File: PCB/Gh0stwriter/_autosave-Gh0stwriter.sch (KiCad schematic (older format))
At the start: 20 parts, among them J1 Conn_01x06, J2 Conn_01x02, J3 Conn_01x06, J4 Conn_01x02, J5 Conn_01x06, J6 Conn_01x06, J7 Conn_01x02, Q1 Q_NPN_Darlington_ECB

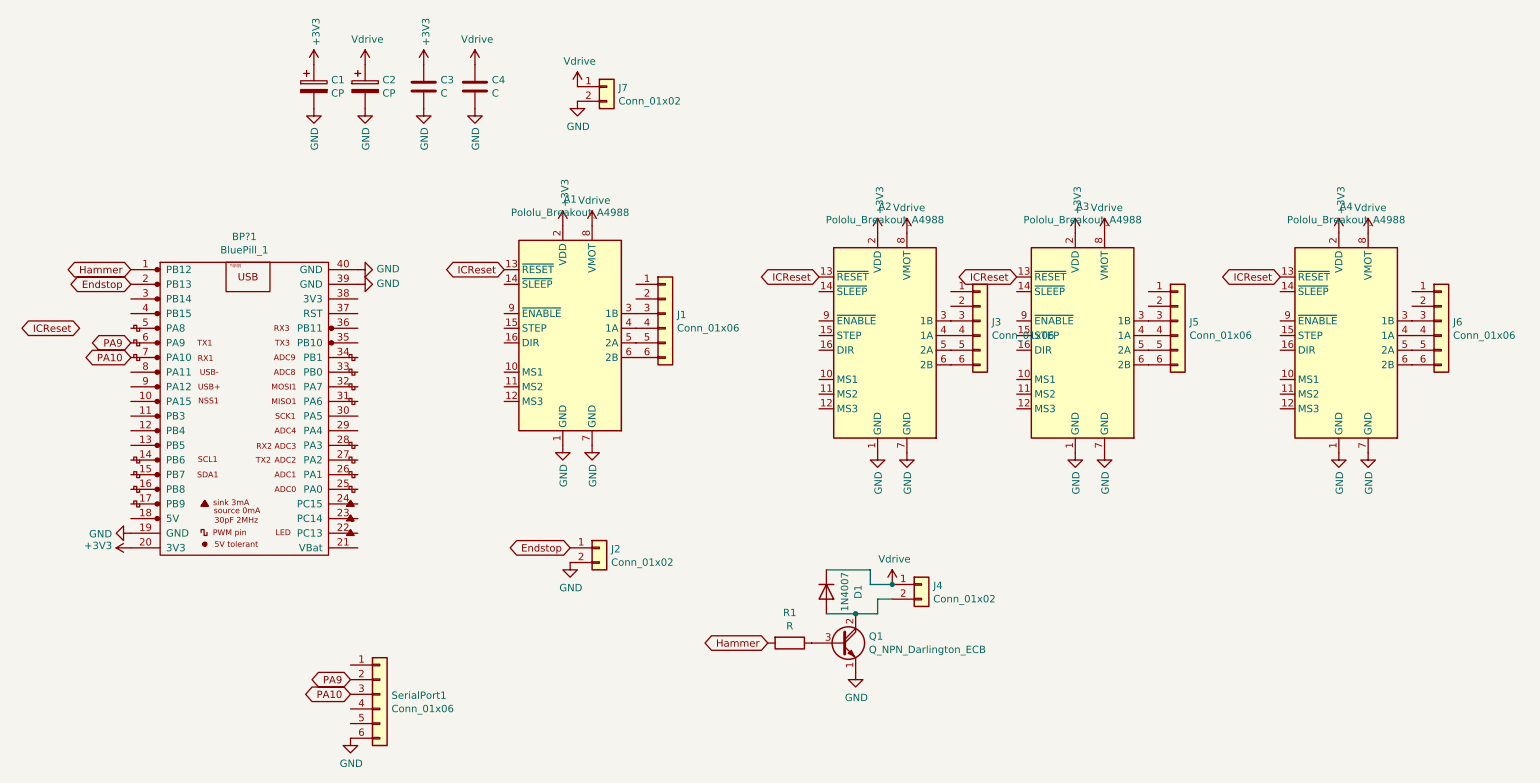
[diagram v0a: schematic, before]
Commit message: Finished first Version of the pcb
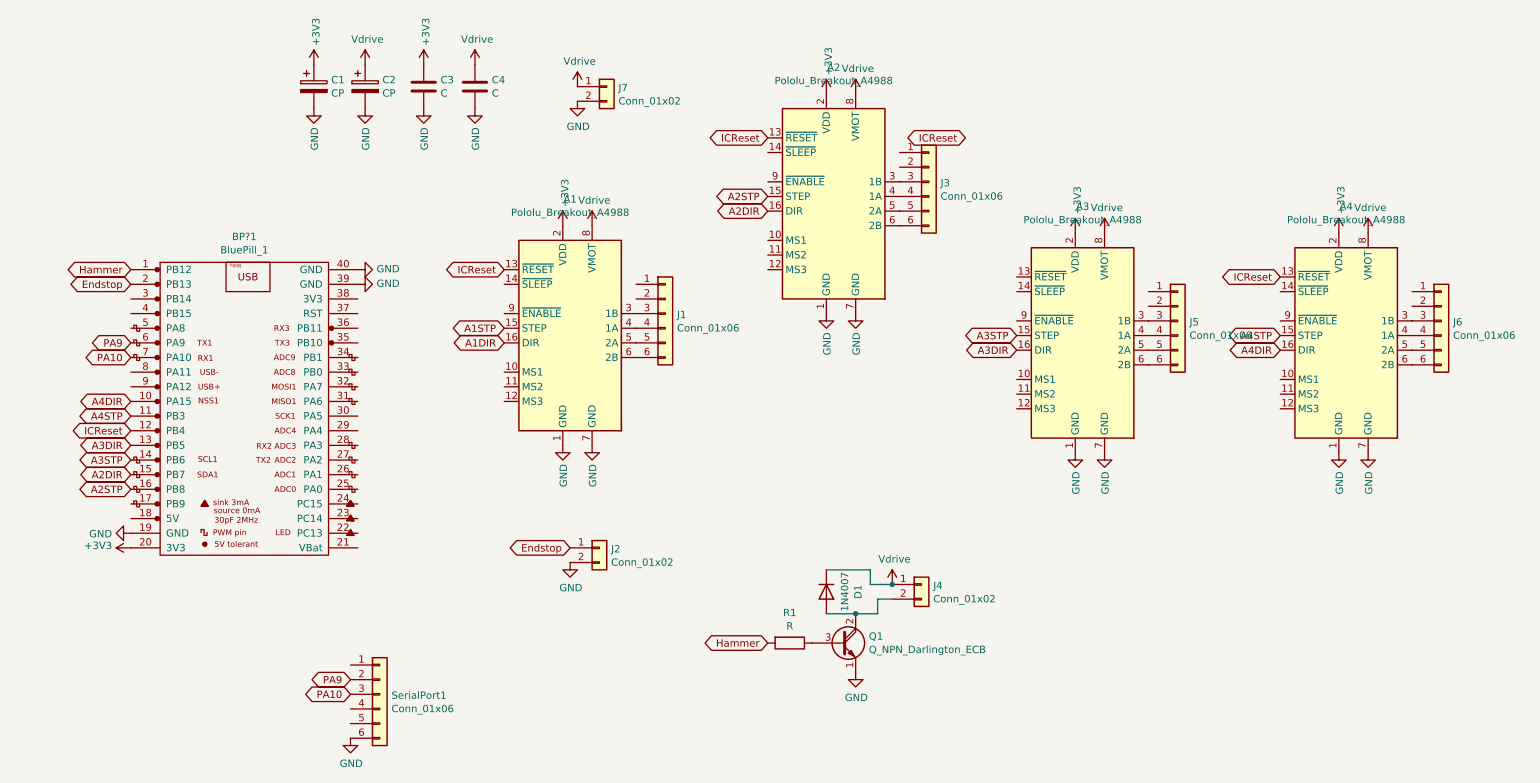
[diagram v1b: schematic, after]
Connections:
- net ICReset: now also BP?1.12 (PB4); no longer A3.13 (~RESET)
- net A3STP: now reaches A3.15 (STEP)
- net A3STP: now also BP?1.14 (PB6)
- net A3DIR: now reaches A3.16 (DIR)
- net A3DIR: now also BP?1.13 (PB5)
- net A4DIR: now reaches BP?1.10 (PA15)
- net A4DIR: now also A4.16 (DIR)
- net A4STP: now reaches BP?1.11 (PB3)
- net A4STP: now also A4.15 (STEP)
- net A2DIR: now reaches BP?1.15 (PB7)
- net A2DIR: now also A2.16 (DIR)
- net A2STP: now reaches BP?1.16 (PB8)
- net A2STP: now also A2.15 (STEP)
- net A1STP: now reaches A1.15 (STEP)
- net A1DIR: now reaches A1.16 (DIR)
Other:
- moved on the sheet: A2, J3
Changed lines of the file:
@@
 L Driver_Motor:Pololu_Breakout_A4988 A2
 U 1 1 5ECFA6AE
-P 6250 4250
-F 0 "A2" H 6300 5131 50  0000 C CNN
-F 1 "Pololu_Breakout_A4988" H 6300 5040 50  0000 C CNN
-F 2 "Module:Pololu_Breakout-16_15.2x20.3mm" H 6525 3500 50  0001 L CNN
-F 3 "https://www.pololu.com/product/2980/pictures" H 6350 3950 50  0001 C CNN
-	1    6250 4250
+P 5900 3300
+F 0 "A2" H 5950 4181 50  0000 C CNN
+F 1 "Pololu_Breakout_A4988" H 5950 4090 50  0000 C CNN
+F 2 "Module:Pololu_Breakout-16_15.2x20.3mm" H 6175 2550 50  0001 L CNN
+F 3 "https://www.pololu.com/product/2980/pictures" H 6000 3000 50  0001 C CNN
+	1    5900 3300
 	1    0    0    -1
 $EndComp
@@
 L power:GND #PWR0111
 U 1 1 5ED7A1C8
-P 6250 5050
-F 0 "#PWR0111" H 6250 4800 50  0001 C CNN
-F 1 "GND" V 6255 4922 50  0000 R CNN
-F 2 "" H 6250 5050 50  0001 C CNN
-F 3 "" H 6250 5050 50  0001 C CNN
-	1    6250 5050
+P 5900 4100
+F 0 "#PWR0111" H 5900 3850 50  0001 C CNN
+F 1 "GND" V 5905 3972 50  0000 R CNN
+F 2 "" H 5900 4100 50  0001 C CNN
+F 3 "" H 5900 4100 50  0001 C CNN
+	1    5900 4100
 	1    0    0    -1
 $EndComp
@@
 L power:GND #PWR0112
 U 1 1 5ED7A4BD
-P 6450 5050
-F 0 "#PWR0112" H 6450 4800 50  0001 C CNN
-F 1 "GND" V 6455 4922 50  0000 R CNN
-F 2 "" H 6450 5050 50  0001 C CNN
-F 3 "" H 6450 5050 50  0001 C CNN
-	1    6450 5050
+P 6100 4100
+F 0 "#PWR0112" H 6100 3850 50  0001 C CNN
+F 1 "GND" V 6105 3972 50  0000 R CNN
+F 2 "" H 6100 4100 50  0001 C CNN
+F 3 "" H 6100 4100 50  0001 C CNN
+	1    6100 4100
 	1    0    0    -1
 $EndComp
@@
 L power:+3V3 #PWR0118
 U 1 1 5ED85A0B
-P 6250 3550
-F 0 "#PWR0118" H 6250 3400 50  0001 C CNN
-F 1 "+3V3" V 6265 3678 50  0000 L CNN
-F 2 "" H 6250 3550 50  0001 C CNN
-F 3 "" H 6250 3550 50  0001 C CNN
-	1    6250 3550
+P 5900 2600
+F 0 "#PWR0118" H 5900 2450 50  0001 C CNN
+F 1 "+3V3" V 5915 2728 50  0000 L CNN
+F 2 "" H 5900 2600 50  0001 C CNN
+F 3 "" H 5900 2600 50  0001 C CNN
+	1    5900 2600
 	1    0    0    -1
 $EndComp
@@
 L power:Vdrive #PWR0124
 U 1 1 5EDBB3D5
-P 6450 3550
-F 0 "#PWR0124" H 6250 3400 50  0001 C CNN
-F 1 "Vdrive" H 6465 3723 50  0000 C CNN
-F 2 "" H 6450 3550 50  0001 C CNN
-F 3 "" H 6450 3550 50  0001 C CNN
-	1    6450 3550
+P 6100 2600
+F 0 "#PWR0124" H 5900 2450 50  0001 C CNN
+F 1 "Vdrive" H 6115 2773 50  0000 C CNN
+F 2 "" H 6100 2600 50  0001 C CNN
+F 3 "" H 6100 2600 50  0001 C CNN
+	1    6100 2600
 	1    0    0    -1
 $EndComp
@@
 Text GLabel 3700 3800 0    50   BiDi ~ 0
 ICReset
-Text GLabel 5850 3850 0    50   BiDi ~ 0
+Text GLabel 5500 2900 0    50   BiDi ~ 0
 ICReset
-Text GLabel 7200 3850 0    50   BiDi ~ 0
+Text GLabel 6850 2900 0    50   BiDi ~ 0
 ICReset
 Text GLabel 9000 3850 0    50   BiDi ~ 0
 ICReset
-Text GLabel 800  4200 0    50   BiDi ~ 0
+Text GLabel 1150 4900 0    50   BiDi ~ 0
 ICReset
 $Comp
 L Connector_Generic:Conn_01x06 J3
 U 1 1 5EE5F861
-P 6950 4150
-F 0 "J3" H 7030 4142 50  0000 L CNN
-F 1 "Conn_01x06" H 7030 4051 50  0000 L CNN
-F 2 "Connector_JST:JST_XH_B6B-XH-A_1x06_P2.50mm_Vertical" H 6950 4150 50  0001 C CNN
-F 3 "~" H 6950 4150 50  0001 C CNN
-	1    6950 4150
+P 6600 3200
+F 0 "J3" H 6680 3192 50  0000 L CNN
+F 1 "Conn_01x06" H 6680 3101 50  0000 L CNN
+F 2 "Connector_JST:JST_XH_B6B-XH-A_1x06_P2.50mm_Vertical" H 6600 3200 50  0001 C CNN
+F 3 "~" H 6600 3200 50  0001 C CNN
+	1    6600 3200
 	1    0    0    -1
 $EndComp
@@
 Text GLabel 1150 3900 0    50   BiDi ~ 0
 Endstop
+Text GLabel 1150 4700 0    50   BiDi ~ 0
+A4DIR
+Text GLabel 1150 4800 0    50   BiDi ~ 0
+A4STP
+Text GLabel 9000 4250 0    50   BiDi ~ 0
+A4STP
+Text GLabel 9000 4350 0    50   BiDi ~ 0
+A4DIR
+Text GLabel 7200 4250 0    50   BiDi ~ 0
+A3STP
+Text GLabel 7200 4350 0    50   BiDi ~ 0
+A3DIR
+Text GLabel 5500 3300 0    50   BiDi ~ 0
+A2STP
+Text GLabel 5500 3400 0    50   BiDi ~ 0
+A2DIR
+Text GLabel 3700 4200 0    50   BiDi ~ 0
+A1STP
+Text GLabel 3700 4300 0    50   BiDi ~ 0
+A1DIR
+Text GLabel 1150 5000 0    50   BiDi ~ 0
+A3DIR
+Text GLabel 1150 5100 0    50   BiDi ~ 0
+A3STP
+Text GLabel 1150 5200 0    50   BiDi ~ 0
+A2DIR
+Text GLabel 1150 5300 0    50   BiDi ~ 0
+A2STP
 $EndSCHEMATC
